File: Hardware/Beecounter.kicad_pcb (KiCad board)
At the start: 2 copper layers, 171 parts, among them J1 Conn_01x03, J10 Conn_01x03, J11 Conn_01x03, J12 Conn_01x03, J13 Conn_01x03, J14 Conn_01x03, J15 Conn_02x20_Odd_Even, J16 Conn_01x04, J17 Conn_01x10, J2 Conn_01x03, J3 Conn_01x03, J4 Conn_01x03, J5 Conn_01x03, J6 Conn_01x03, J7 Conn_01x03, J8 Conn_01x03, J9 Conn_01x03, U1 LM393, U10 LM393, U11 H2010, U12 LM393, U13 H2010, U14 LM393, U15 H2010, U16 LM393, U17 H2010, U18 LM393, U19 H2010, U2 H2010, U20 LM393, U21 H2010, U22 LM393, U23 H2010, U24 LM393, U25 H2010, U26 LM393, U27 H2010, U28 LM393, U3 H2010, U4 LM393, U5 H2010, U6 LM393, U7 H2010, U8 LM393, U9 H2010

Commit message: Generated GND area and Gerber files
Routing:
- added copper zone on B.Cu, net GND
- removed copper zone on B.Cu, net (none)
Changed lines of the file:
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@@
 		(min_thickness 0.25)
 		(filled_areas_thickness no)
-		(fill
+		(fill yes
 			(thermal_gap 0.5)
 			(thermal_bridge_width 0.5)
@@
 	)
 	(zone
-		(net 0)
-		(net_name "")
+		(net 2)
+		(net_name "GND")
 		(layer "B.Cu")
 		(name "GND B.Cu")
@@
 		(min_thickness 0.25)
 		(filled_areas_thickness no)
-		(fill
+		(fill yes
 			(thermal_gap 0.5)
 			(thermal_bridge_width 0.5)

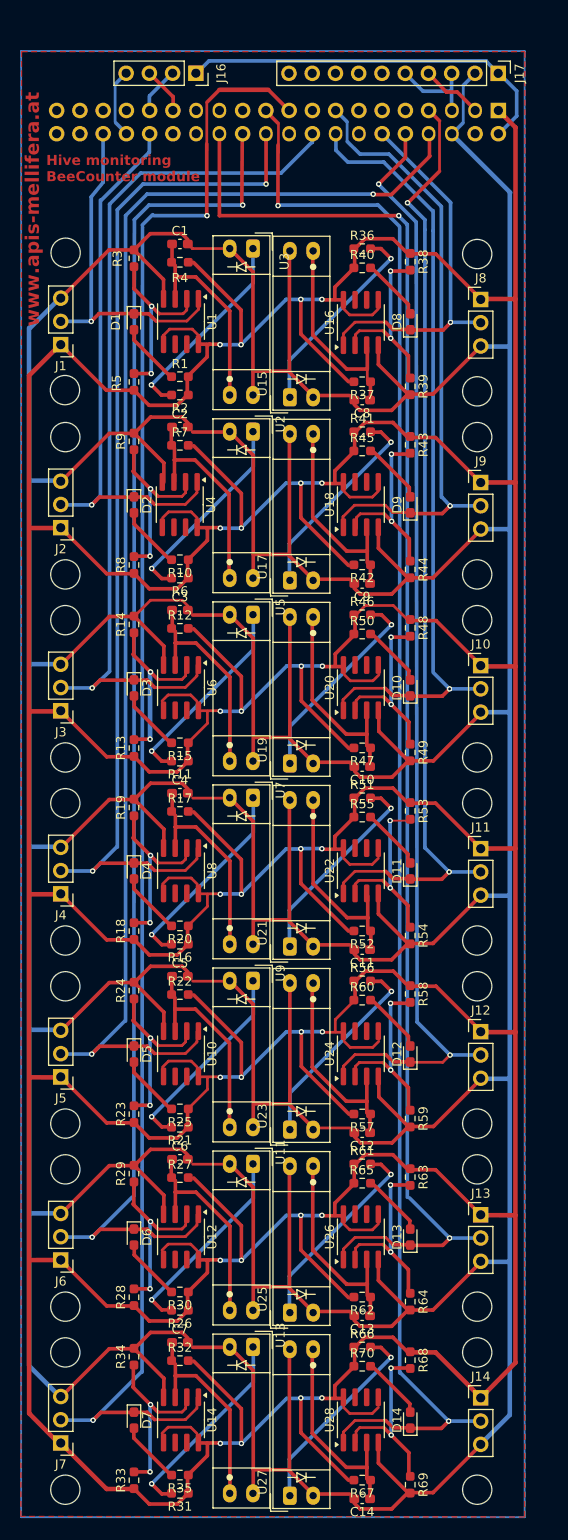
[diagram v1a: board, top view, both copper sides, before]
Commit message: Set origin
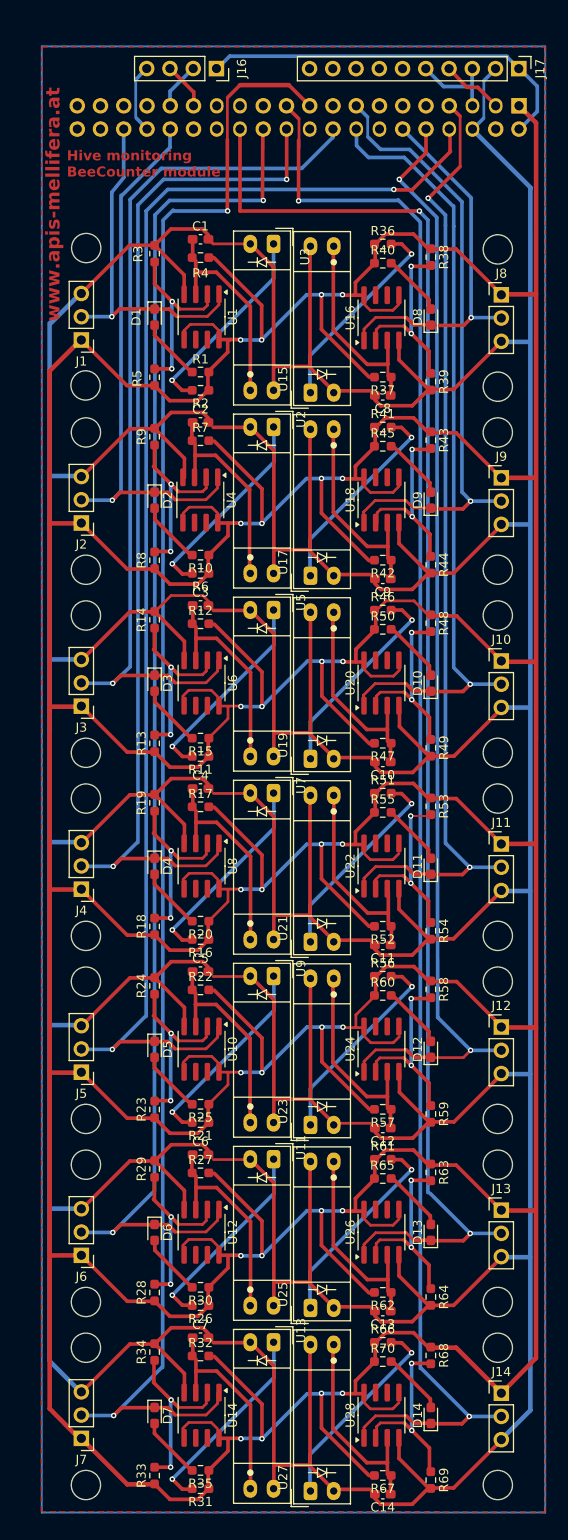
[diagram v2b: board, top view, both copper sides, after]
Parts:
- moved R56 2.31 mm to (77.2, 141.4)
- moved R60 2.31 mm to (77.2, 143.5)
- moved R61 2.31 mm to (77.2, 161.4)
- moved R65 2.31 mm to (77.2, 163.5)
- moved R66 2.31 mm to (77.2, 181.4)
- moved R70 2.31 mm to (77.2, 183.5)
- moved ? 2.31 mm to (89.8, 97.0)
- moved ? 2.31 mm to (44.8, 82.0)
- moved ? 2.31 mm to (44.8, 102.0)
- moved ? 2.31 mm to (89.8, 102.0)
- moved ? 2.31 mm to (89.8, 82.0)
- moved ? 2.31 mm to (89.8, 122.0)
- moved ? 2.31 mm to (89.8, 62.0)
- moved ? 2.31 mm to (44.8, 97.0)
- moved ? 2.31 mm to (89.8, 117.0)
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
